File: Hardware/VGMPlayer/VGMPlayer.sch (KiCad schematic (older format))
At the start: 75 parts, among them J1 USB_B_Mini, J2 SD_Card, SW1 Play/Suffle, SW2 Stop, SW3 Next/Pause, SW4 Prev/Resume, U1 STM32F103XX, U10 LTC6903, U11 HC-06, U13 YM3012, U14 LM324, U18 OLED_128_64_I2C, U19 ESP8266Module, U3 LM386, U4 LM386, U5 YM2151, U6 AUDIOJACK-VGM, U7 YM2612, U8 SN76489, U9 LTC6903

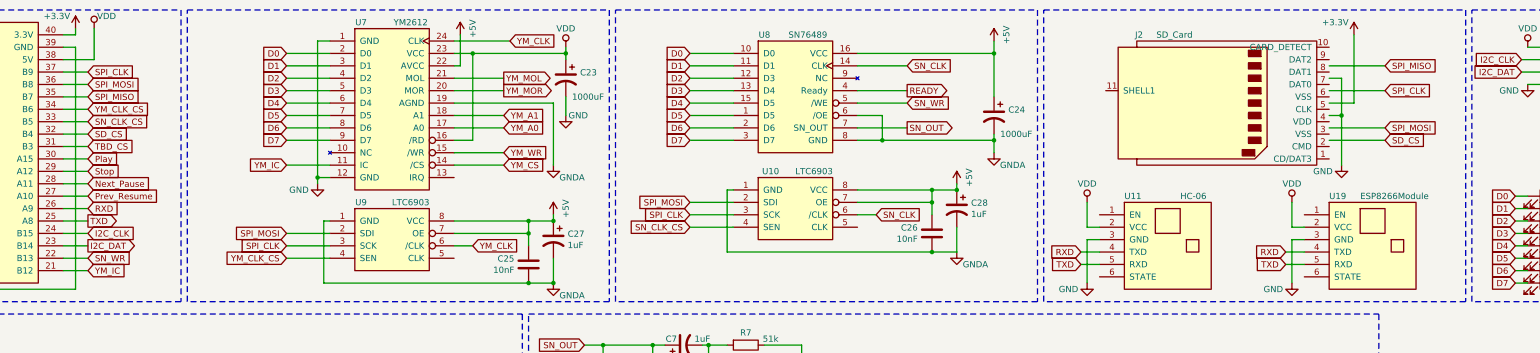
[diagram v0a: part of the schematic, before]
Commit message: 1
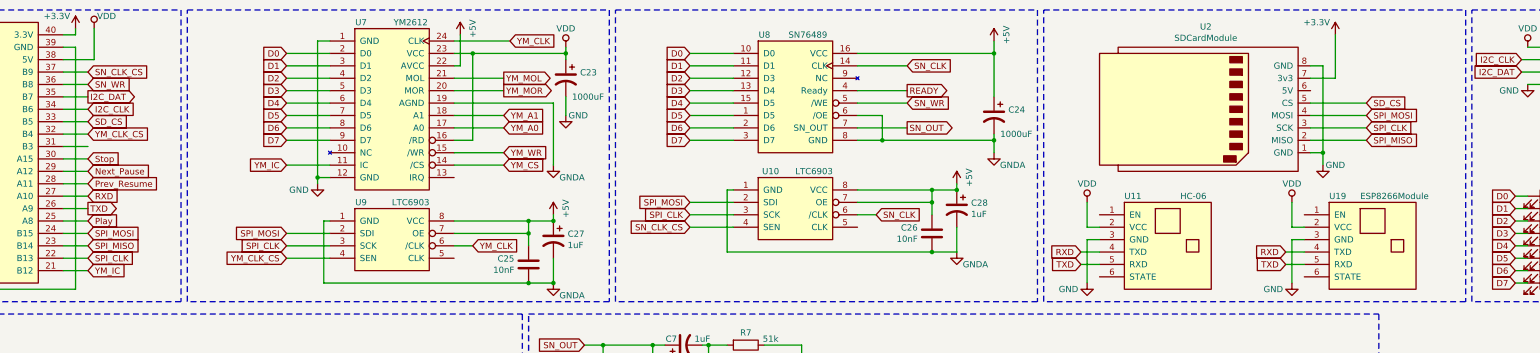
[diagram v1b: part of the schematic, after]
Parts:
- removed J2: SD_Card, Connector_Card:SD_TE_2041021, symbol VGMPlayer-rescue:SD_Card
- added U2: SDCardModule, Connector_PinHeader_2.54mm:PinHeader_1x08_P2.54mm_Vertical, symbol VGMPlayer-rescue:SDCardModule
- D1, D2, D3, D4, D5, D6, D7, D8: footprint (none) -> LED_SMD:LED_0805_2012Metric
- RV1, RV2: footprint Varistor:RV_Disc_D7mm_W3.4mm_P5mm -> Connector_PinHeader_2.54mm:PinHeader_1x03_P2.54mm_Vertical
- SW1, SW2, SW3, SW4: footprint (none) -> Button_Switch_THT:SW_Tactile_Straight_KSA0Axx1LFTR
- U1: footprint Package_DIP:DIP-40_W25.4mm_Socket -> Package_DIP:DIP-40_W15.24mm_Socket
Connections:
- net +3V3: now also U2.7 (3v3)
- net GND: now also U2.1 (GND), U2.8 (GND)
- net I2C_CLK: now also U1.34 (B6); no longer U1.24 (B15)
- net I2C_DAT: now also U1.35 (B7); no longer U1.23 (B14)
- net Next_Pause: now also U1.29 (A12); no longer U1.28 (A11)
- net Play: now also U1.25 (A8); no longer U1.30 (A15)
- net Prev_Resume: now also U1.28 (A11); no longer U1.27 (A10)
- net RXD: now also U1.27 (A10); no longer U1.26 (A9)
- net SD_CS: now also U1.33 (B5), U2.5 (CS); no longer U1.32 (B4)
- net SN_CLK_CS: now also U1.37 (B9); no longer U1.33 (B5)
- net SN_WR: now also U1.36 (B8); no longer U1.22 (B13)
- net SPI_CLK: now also U1.22 (B13), U2.3 (SCK); no longer U1.37 (B9)
- net SPI_MISO: now also U1.23 (B14), U2.2 (MISO); no longer U1.35 (B7)
- net SPI_MOSI: now also U1.24 (B15), U2.4 (MOSI); no longer U1.36 (B8)
- net Stop: now also U1.30 (A15); no longer U1.29 (A12)
- net TXD: now also U1.26 (A9); no longer U1.25 (A8)
- net YM_CLK_CS: now also U1.32 (B4); no longer U1.34 (B6)
- net TBD_CS: no longer names the net of U1.31 (B3)
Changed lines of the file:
@@
 Text GLabel 2300 2250 0    50   Input ~ 0
 YM_A1
-Text GLabel 4050 1250 2    50   Input ~ 0
+Text GLabel 4050 2450 2    50   Input ~ 0
 SPI_MISO
+Text GLabel 4050 2550 2    50   Input ~ 0
+SPI_CLK
+Text GLabel 4050 2350 2    50   Input ~ 0
+SPI_MOSI
+Text GLabel 4050 1550 2    50   Input ~ 0
+YM_CLK_CS
 Text GLabel 4050 1050 2    50   Input ~ 0
-SPI_CLK
-Text GLabel 4050 1150 2    50   Input ~ 0
-SPI_MOSI
-Text GLabel 4050 1350 2    50   Input ~ 0
-YM_CLK_CS
-Text GLabel 4050 1450 2    50   Input ~ 0
 SN_CLK_CS
 $Comp
@@
 Wire Wire Line
 	7100 4100 7100 4200
-Text GLabel 4050 1550 2    50   Input ~ 0
+Text GLabel 4050 1450 2    50   Input ~ 0
 SD_CS
-Text GLabel 4050 1650 2    50   Input ~ 0
-TBD_CS
-Text GLabel 4050 2550 2    50   Input ~ 0
+Text GLabel 4050 1150 2    50   Input ~ 0
 SN_WR
 Wire Wire Line
@@
 F 0 "U1" H 2700 700 50  0000 C CNN
 F 1 "STM32F103XX" H 3050 700 50  0000 C CNN
-F 2 "Package_DIP:DIP-40_W25.4mm_Socket" H 3100 700 50  0001 C CNN
+F 2 "Package_DIP:DIP-40_W15.24mm_Socket" H 3100 700 50  0001 C CNN
 F 3 "" H 3100 700 50  0001 C CNN
 	1    3100 650
@@
 Wire Wire Line
 	4100 950  3850 950
-Text GLabel 4050 2350 2    50   Input ~ 0
+Text GLabel 4050 1350 2    50   Input ~ 0
 I2C_CLK
-Text GLabel 4050 2450 2    50   Output ~ 0
+Text GLabel 4050 1250 2    50   Output ~ 0
 I2C_DAT
-Text GLabel 4050 2150 2    50   Input ~ 0
+Text GLabel 4050 2050 2    50   Input ~ 0
 RXD
-Text GLabel 4050 2250 2    50   Output ~ 0
+Text GLabel 4050 2150 2    50   Output ~ 0
 TXD
 $Comp
@@
 F 0 "RV1" H 9982 6546 50  0000 R CNN
 F 1 "10k" H 9982 6455 50  0000 R CNN
-F 2 "Varistor:RV_Disc_D7mm_W3.4mm_P5mm" H 10050 6500 50  0001 C CNN
+F 2 "Connector_PinHeader_2.54mm:PinHeader_1x03_P2.54mm_Vertical" H 10050 6500 50  0001 C CNN
 F 3 "~" H 10050 6500 50  0001 C CNN
 	1    10050 6500
@@
 F 0 "RV2" H 9982 5046 50  0000 R CNN
 F 1 "10k" H 9982 4955 50  0000 R CNN
-F 2 "Varistor:RV_Disc_D7mm_W3.4mm_P5mm" H 10050 5000 50  0001 C CNN
+F 2 "Connector_PinHeader_2.54mm:PinHeader_1x03_P2.54mm_Vertical" H 10050 5000 50  0001 C CNN
 F 3 "~" H 10050 5000 50  0001 C CNN
 	1    10050 5000
@@
 Wire Wire Line
 	10050 5150 10050 5200
-$Comp
-L VGMPlayer-rescue:SD_Card J2
-U 1 1 5F3D5C10
-P 13150 1300
-F 0 "J2" H 13750 750 50  0000 L CNN
-F 1 "SD_Card" H 13350 750 50  0000 L CNN
-F 2 "Connector_Card:SD_TE_2041021" H 13150 1300 50  0001 C CNN
-F 3 "http://portal.fciconnect.com/Comergent//fci/drawing/10067847.pdf" H 13150 1300 50  0001 C CNN
-	1    13150 1300
-	-1   0    0    1
-$EndComp
 Wire Notes Line
 	15200 550  18600 550
@@
 Wire Notes Line
 	18600 2900 15200 2900
-Text GLabel 14500 1000 2    50   Input ~ 0
+Text GLabel 14350 1600 2    50   Input ~ 0
 SPI_MISO
-Text GLabel 14500 1500 2    50   Input ~ 0
+Text GLabel 14350 1400 2    50   Input ~ 0
 SPI_MOSI
-Text GLabel 14500 1200 2    50   Input ~ 0
+Text GLabel 14350 1500 2    50   Input ~ 0
 SPI_CLK
-Text GLabel 14500 1600 2    50   Input ~ 0
+Text GLabel 14350 1300 2    50   Input ~ 0
 SD_CS
 $Comp
 L power:GND #PWR027
 U 1 1 5F546118
-P 14150 1800
-F 0 "#PWR027" H 14150 1550 50  0001 C CNN
-F 1 "GND" H 14000 1750 50  0000 C CNN
-F 2 "" H 14150 1800 50  0001 C CNN
-F 3 "" H 14150 1800 50  0001 C CNN
-	1    14150 1800
+P 14000 1800
+F 0 "#PWR027" H 14000 1550 50  0001 C CNN
+F 1 "GND" H 14100 1800 50  0000 C CNN
+F 2 "" H 14000 1800 50  0001 C CNN
+F 3 "" H 14000 1800 50  0001 C CNN
+	1    14000 1800
 	1    0    0    -1
 $EndComp
@@
 L power:+3.3V #PWR028
 U 1 1 5F56EE7E
-P 14250 750
-F 0 "#PWR028" H 14250 600 50  0001 C CNN
-F 1 "+3.3V" H 14100 850 50  0000 C CNN
-F 2 "" H 14250 750 50  0001 C CNN
-F 3 "" H 14250 750 50  0001 C CNN
-	1    14250 750
-	1    0    0    -1
-$EndComp
-Wire Wire Line
-	14050 1400 14150 1400
-Wire Wire Line
-	14150 1400 14150 1100
-Wire Wire Line
-	14500 1200 14050 1200
-Wire Wire Line
-	14500 1600 14050 1600
-Wire Wire Line
-	14050 1500 14500 1500
-Wire Wire Line
-	14050 1000 14500 1000
-Wire Wire Line
-	14050 1300 14250 1300
-Connection ~ 14150 1400
-Wire Wire Line
-	14150 1100 14050 1100
-Wire Wire Line
-	14250 750  14250 1300
-Wire Wire Line
-	14150 1800 14150 1400
+P 14100 750
+F 0 "#PWR028" H 14100 600 50  0001 C CNN
+F 1 "+3.3V" H 13950 850 50  0000 C CNN
+F 2 "" H 14100 750 50  0001 C CNN
+F 3 "" H 14100 750 50  0001 C CNN
+	1    14100 750
+	1    0    0    -1
+$EndComp
+Wire Wire Line
+	13900 1700 14000 1700
+Wire Wire Line
+	14350 1500 13900 1500
+Wire Wire Line
+	14350 1300 13900 1300
+Wire Wire Line
+	13900 1400 14350 1400
+Wire Wire Line
+	13900 1600 14350 1600
+Wire Wire Line
+	13900 1100 14100 1100
+Wire Wire Line
+	14000 1000 13900 1000
+Wire Wire Line
+	14100 750  14100 1100
+Wire Wire Line
+	14000 1800 14000 1700
 Wire Wire Line
 	11650 6250 11900 6250
@@
 F 0 "SW1" H 18050 1685 50  0000 C CNN
 F 1 "Play/Suffle" H 18050 1594 50  0000 C CNN
-F 2 "" H 18050 1600 50  0001 C CNN
+F 2 "Button_Switch_THT:SW_Tactile_Straight_KSA0Axx1LFTR" H 18050 1600 50  0001 C CNN
 F 3 "" H 18050 1600 50  0001 C CNN
 	1    18050 1400
@@
 F 0 "SW2" H 18050 2085 50  0000 C CNN
 F 1 "Stop" H 18050 1994 50  0000 C CNN
-F 2 "" H 18050 2000 50  0001 C CNN
+F 2 "Button_Switch_THT:SW_Tactile_Straight_KSA0Axx1LFTR" H 18050 2000 50  0001 C CNN
 F 3 "" H 18050 2000 50  0001 C CNN
 	1    18050 1800
@@
 F 0 "SW3" H 18050 2485 50  0000 C CNN
 F 1 "Next/Pause" H 18050 2394 50  0000 C CNN
-F 2 "" H 18050 2400 50  0001 C CNN
+F 2 "Button_Switch_THT:SW_Tactile_Straight_KSA0Axx1LFTR" H 18050 2400 50  0001 C CNN
 F 3 "" H 18050 2400 50  0001 C CNN
 	1    18050 2200
@@
 F 0 "SW4" H 18050 2885 50  0000 C CNN
 F 1 "Prev/Resume" H 18050 2794 50  0000 C CNN
-F 2 "" H 18050 2800 50  0001 C CNN
+F 2 "Button_Switch_THT:SW_Tactile_Straight_KSA0Axx1LFTR" H 18050 2800 50  0001 C CNN
 F 3 "" H 18050 2800 50  0001 C CNN
 	1    18050 2600
@@
 Wire Wire Line
 	17850 2600 17750 2600
+Text GLabel 4050 2250 2    50   Input ~ 0
+Play
 Text GLabel 4050 1750 2    50   Input ~ 0
-Play
+Stop
 Text GLabel 4050 1850 2    50   Input ~ 0
-Stop
+Next_Pause
 Text GLabel 4050 1950 2    50   Input ~ 0
-Next_Pause
-Text GLabel 4050 2050 2    50   Input ~ 0
 Prev_Resume
 Wire Wire Line
@@
 F 0 "D1" H 15900 2000 50  0000 C CNN
 F 1 "LED" H 15950 2100 50  0001 C CNN
-F 2 "" H 15800 2050 50  0001 C CNN
+F 2 "LED_SMD:LED_0805_2012Metric" H 15800 2050 50  0001 C CNN
 F 3 "~" H 15800 2050 50  0001 C CNN
 	1    15800 2050
@@
 F 0 "D2" H 15900 2100 50  0000 C CNN
 F 1 "LED" H 15950 2200 50  0001 C CNN
-F 2 "" H 15800 2150 50  0001 C CNN
+F 2 "LED_SMD:LED_0805_2012Metric" H 15800 2150 50  0001 C CNN
 F 3 "~" H 15800 2150 50  0001 C CNN
 	1    15800 2150
@@
 F 0 "D3" H 15900 2200 50  0000 C CNN
 F 1 "LED" H 15950 2300 50  0001 C CNN
-F 2 "" H 15800 2250 50  0001 C CNN
+F 2 "LED_SMD:LED_0805_2012Metric" H 15800 2250 50  0001 C CNN
 F 3 "~" H 15800 2250 50  0001 C CNN
 	1    15800 2250
@@
 F 0 "D4" H 15900 2300 50  0000 C CNN
 F 1 "LED" H 15950 2400 50  0001 C CNN
-F 2 "" H 15800 2350 50  0001 C CNN
+F 2 "LED_SMD:LED_0805_2012Metric" H 15800 2350 50  0001 C CNN
 F 3 "~" H 15800 2350 50  0001 C CNN
 	1    15800 2350
@@
 F 0 "D5" H 15900 2400 50  0000 C CNN
 F 1 "LED" H 15950 2500 50  0001 C CNN
-F 2 "" H 15800 2450 50  0001 C CNN
+F 2 "LED_SMD:LED_0805_2012Metric" H 15800 2450 50  0001 C CNN
 F 3 "~" H 15800 2450 50  0001 C CNN
 	1    15800 2450
@@
 F 0 "D6" H 15900 2500 50  0000 C CNN
 F 1 "LED" H 15950 2600 50  0001 C CNN
-F 2 "" H 15800 2550 50  0001 C CNN
+F 2 "LED_SMD:LED_0805_2012Metric" H 15800 2550 50  0001 C CNN
 F 3 "~" H 15800 2550 50  0001 C CNN
 	1    15800 2550
@@
 F 0 "D7" H 15900 2600 50  0000 C CNN
 F 1 "LED" H 15950 2700 50  0001 C CNN
-F 2 "" H 15800 2650 50  0001 C CNN
+F 2 "LED_SMD:LED_0805_2012Metric" H 15800 2650 50  0001 C CNN
 F 3 "~" H 15800 2650 50  0001 C CNN
 	1    15800 2650
@@
 F 0 "D8" H 15900 2700 50  0000 C CNN
 F 1 "LED" H 15950 2800 50  0001 C CNN
-F 2 "" H 15800 2750 50  0001 C CNN
+F 2 "LED_SMD:LED_0805_2012Metric" H 15800 2750 50  0001 C CNN
 F 3 "~" H 15800 2750 50  0001 C CNN
 	1    15800 2750
@@
 Wire Wire Line
 	16750 2050 15950 2050
+$Comp
+L VGMPlayer-rescue:SDCardModule U2
+U 1 1 5C3D4BB0
+P 12800 1300
+F 0 "U2" H 13056 1915 50  0000 C CNN
+F 1 "SDCardModule" H 13056 1824 50  0000 C CNN
+F 2 "Connector_PinHeader_2.54mm:PinHeader_1x08_P2.54mm_Vertical" H 13050 700 50  0001 C CNN
+F 3 "" H 13050 700 50  0001 C CNN
+	1    12800 1300
+	1    0    0    -1
+$EndComp
+Connection ~ 14000 1700
+Wire Wire Line
+	14000 1000 14000 1700
 $EndSCHEMATC
